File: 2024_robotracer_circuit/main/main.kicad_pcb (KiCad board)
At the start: 2 copper layers, 60 x 60 mm, 69 parts, among them J1 PH_6p, J10 PH_5p, J11 PH_6p, J13 PH_8p, J2 Conn_02x05_Odd_Even, J3 Conn_02x05_Odd_Even, J4 PA_2p, J5 PA_2p, J6 XT_2p, J7 HX_12p, J8 PH_4p, J9 PH_5p, SW1 TVGP01-G73BB, U1 STM32F405RGTx, U10 MTN2306AN3, U16 AE-BMX055, U17 MTN2306AN3, U2 SIT2001B, U22 SKRHAAE010, U23 SS-22F32G5, U3 AM2837, U4 AM2837, U5 BP5293-33, U6 BP5293-50, U7 SSM6J808R, U8 MTN2306AN3

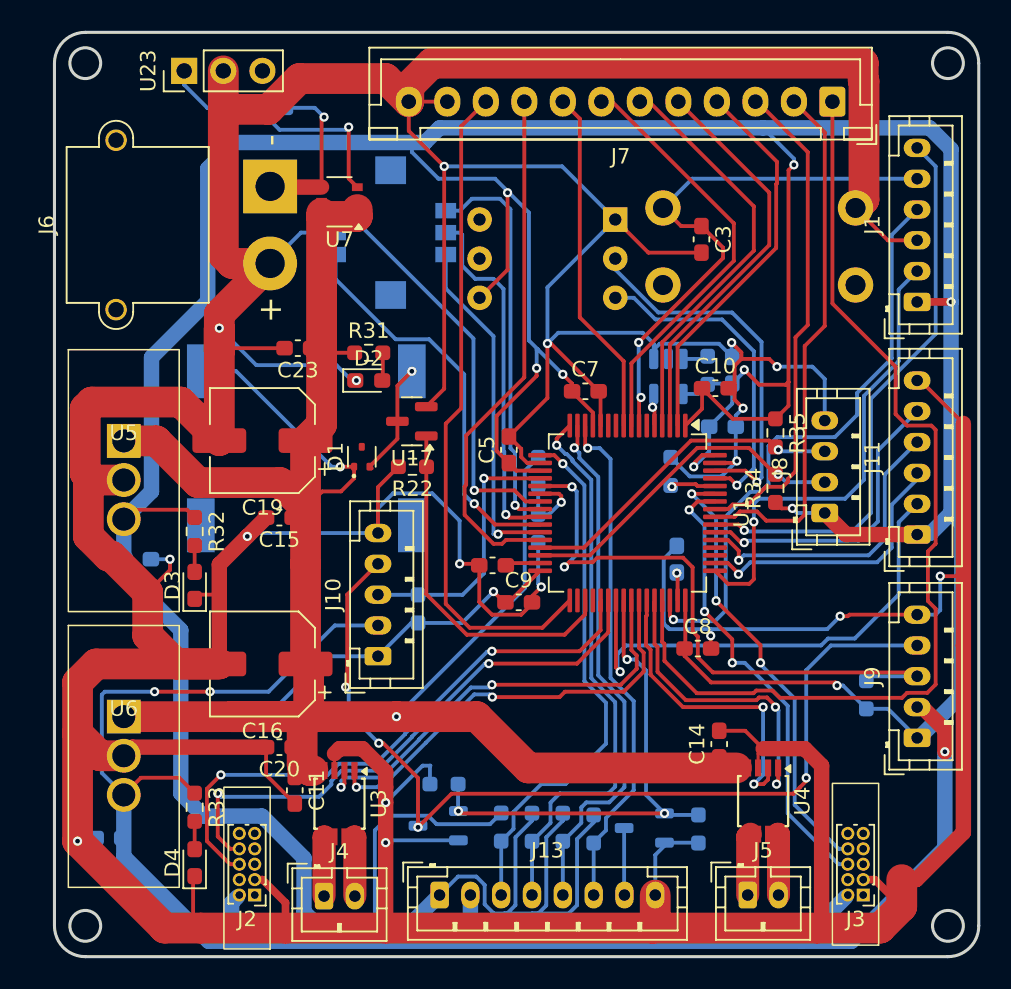
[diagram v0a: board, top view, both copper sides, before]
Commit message: べた
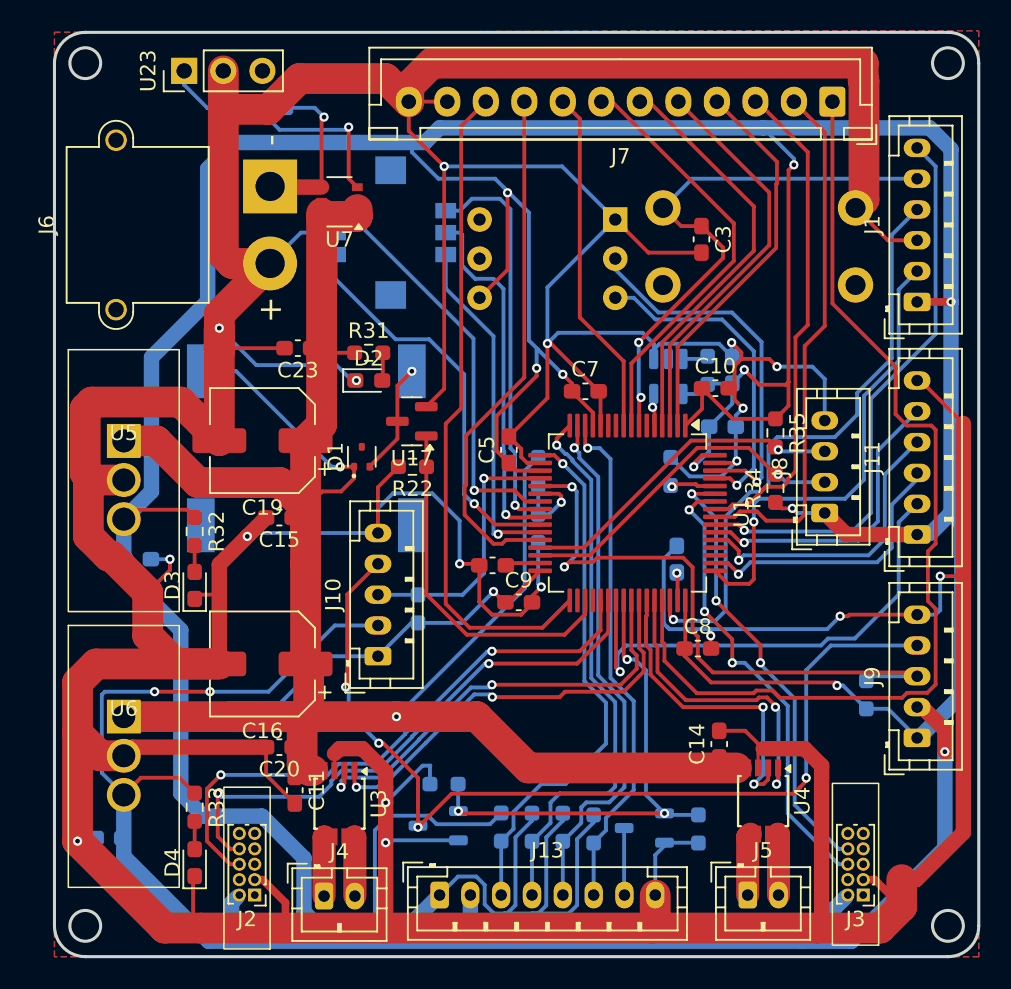
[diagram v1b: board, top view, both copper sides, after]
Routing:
- added copper zone on B.Cu, net GND
- added copper zone on F.Cu, net GND
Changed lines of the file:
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@@
 		(net 87)
+	)
+	(zone
+		(net 2)
+		(net_name "GND")
+		(layers "F&B.Cu")
+		(hatch edge 0.5)
+		(connect_pads
+			(clearance 0.5)
+		)
+		(min_thickness 0.25)
+		(filled_areas_thickness no)
+		(fill yes
+			(thermal_gap 0.5)
+			(thermal_bridge_width 0.5)
+		)
+		(polygon
+			(pts
+				(xy 98 38) (xy 158 37.9) (xy 158 98) (xy 98 98)
+			)
+		)
 	)
 	(group ""
